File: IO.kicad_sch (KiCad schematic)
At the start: 0 parts

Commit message: Transformation in progress
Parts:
- added C4, C5: 4.7nF, Capacitor_SMD:C_0805_2012Metric_Pad1.18x1.45mm_HandSolder, symbol Device:C
- added C6, C7, C8, C9: 0.1μF, symbol Device:C
- added J11: Stop, JST-XH-4A:CONN_B4B-XH-A_JST, symbol JST-XH-4A:B4B-XH-A
- added J6: Hold, JST-XH-2A:CONN_B2B-XH-A_JST, symbol JST-XH-2A:B2B-XH-A
- added J7: X limit, JST-XH-3A:CONN_B3B-XH-A_JST, symbol JST-XH-3A:B3B-XH-A
- added J8: Y limit, JST-XH-3A:CONN_B3B-XH-A_JST, symbol JST-XH-3A:B3B-XH-A
- added R1, R2, R3, R4: 1k, Resistor_SMD:R_0805_2012Metric_Pad1.20x1.40mm_HandSolder, symbol Device:R
- added R10, R11, R12, R9: 100, symbol Device:R
- added R13, R14, R15, R16: 10, symbol Device:R
- added R6: 200, Resistor_SMD:R_0805_2012Metric_Pad1.20x1.40mm_HandSolder, symbol Device:R
- added R7: 1.2k, Resistor_SMD:R_0805_2012Metric_Pad1.20x1.40mm_HandSolder, symbol Device:R
- added SW1: Hold, Button_Switch_THT:SW_SPST_Omron_B3F-40xx, symbol Switch:SW_Push
- added SW2: Run, Button_Switch_THT:SW_SPST_Omron_B3F-40xx, symbol Switch:SW_Push
- added SW3: M1, Button_Switch_THT:SW_SPST_Omron_B3F-40xx, symbol Switch:SW_Push
- added SW4: M2, Button_Switch_THT:SW_SPST_Omron_B3F-40xx, symbol Switch:SW_Push
- added U1: SN74LV125ADR, SN74LV125ADR:SOIC127P600X175-14N, symbol SN74LV125:SN74LV125ADR
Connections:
- new net: R16.1, SW4.2
- new net: R13.2, SW1.2
- new net: R15.1, SW3.2
- new net: R14.2, SW2.2
- new net +5V: U1.1 (1~OE), U1.10 (3~OE), U1.4 (2~OE)
- new net 3.3V: J7.2, R13.1, R14.1, R15.2, R16.2, R6.2, R7.2, U1.14 (VCC)
- new net GND: C4.1, C5.1, C6.1, C7.1, C8.2, C9.2, J11.1, J6.1, J7.1, J8.1, R1.2, R2.2, R3.1, R4.1, U1.7 (GND)
- new net GPIO15: U1.9 (3A)
- new net GPIO2: U1.5 (2A)
- new net GPIO32: C5.2, J8.3, R7.1
- new net GPIO33: J7.3
- new net GPIO34: R10.2
- new net GPIO35: R9.2
- new net GPIO36: R12.2
- new net GPIO39: R11.2
- new net GPIO4: U1.2 (1A)
- new net Hold: C6.2, J6.2, R1.1, R9.1, SW1.1
- new net L_ALARM: J11.4, U1.8 (3Y)
- new net L_HOLD: J11.3, U1.6 (2Y)
- new net L_RUN: J11.2, U1.3 (1Y)
- new net M1: C8.1, R11.1, R3.2, SW3.1
- new net M2: C9.1, R12.1, R4.2, SW4.1
- new net Run: C7.2, R10.1, R2.1, SW2.1
- new net VH: C4.2, J8.2, R6.1
- no-connect marks 0 -> 3

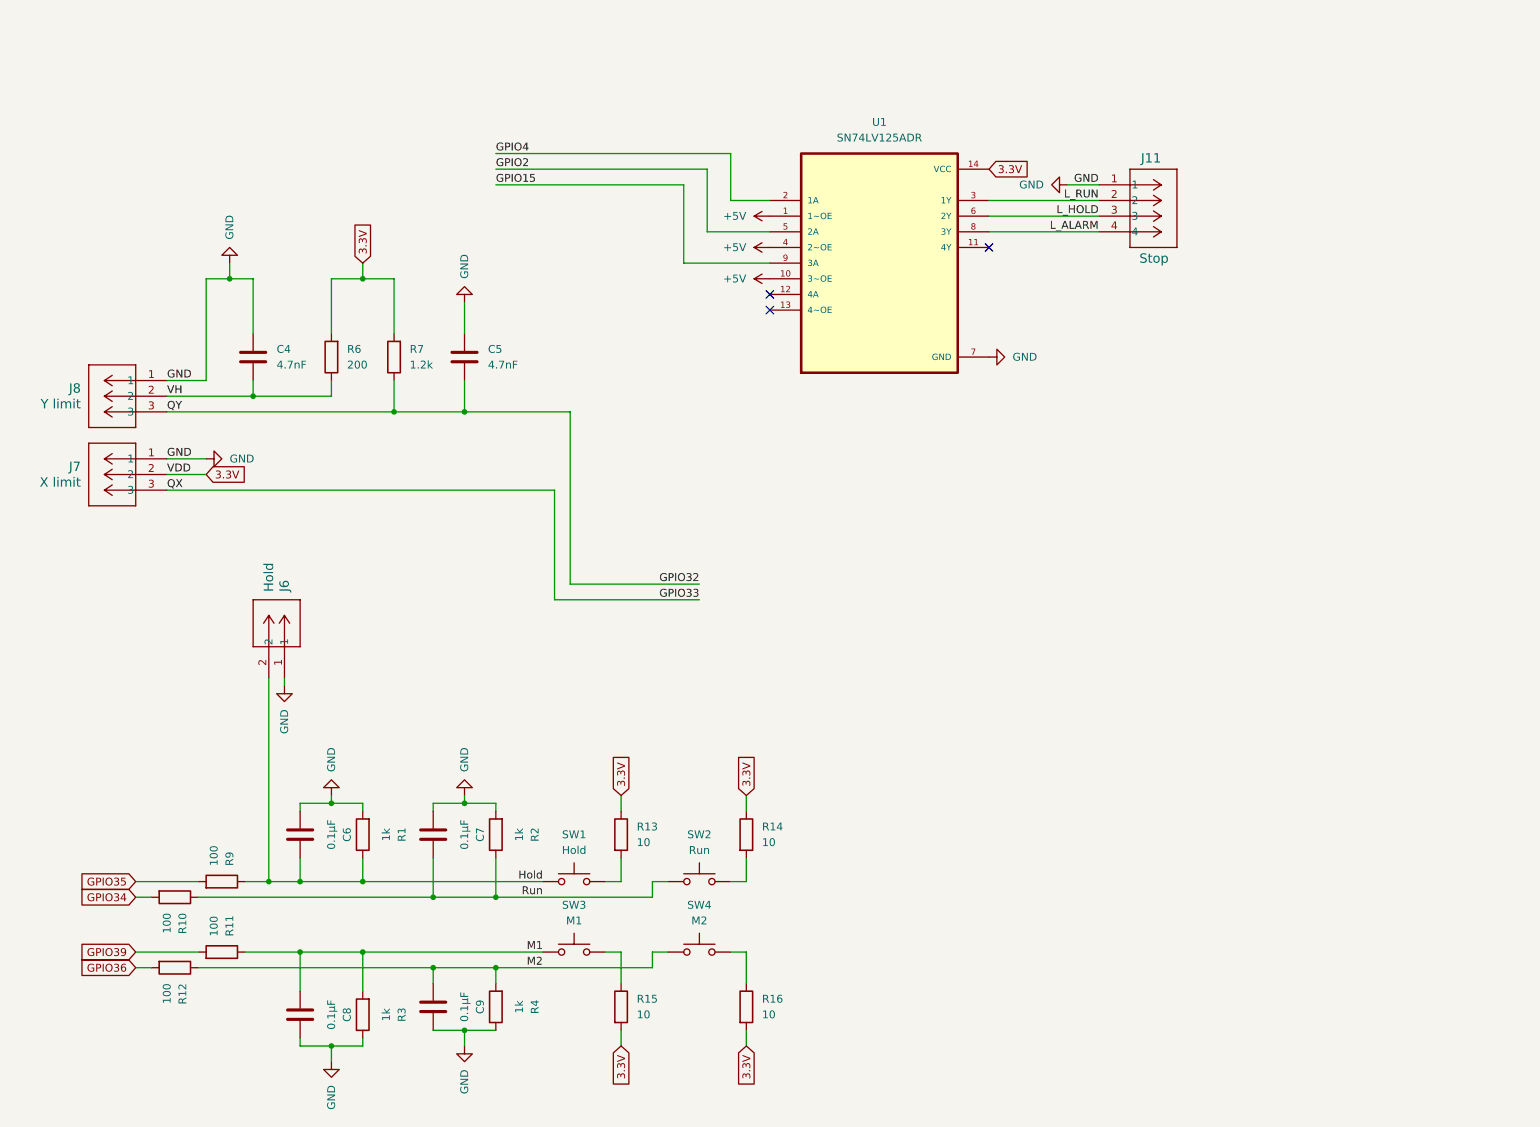
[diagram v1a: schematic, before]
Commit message: Finalization v2.0
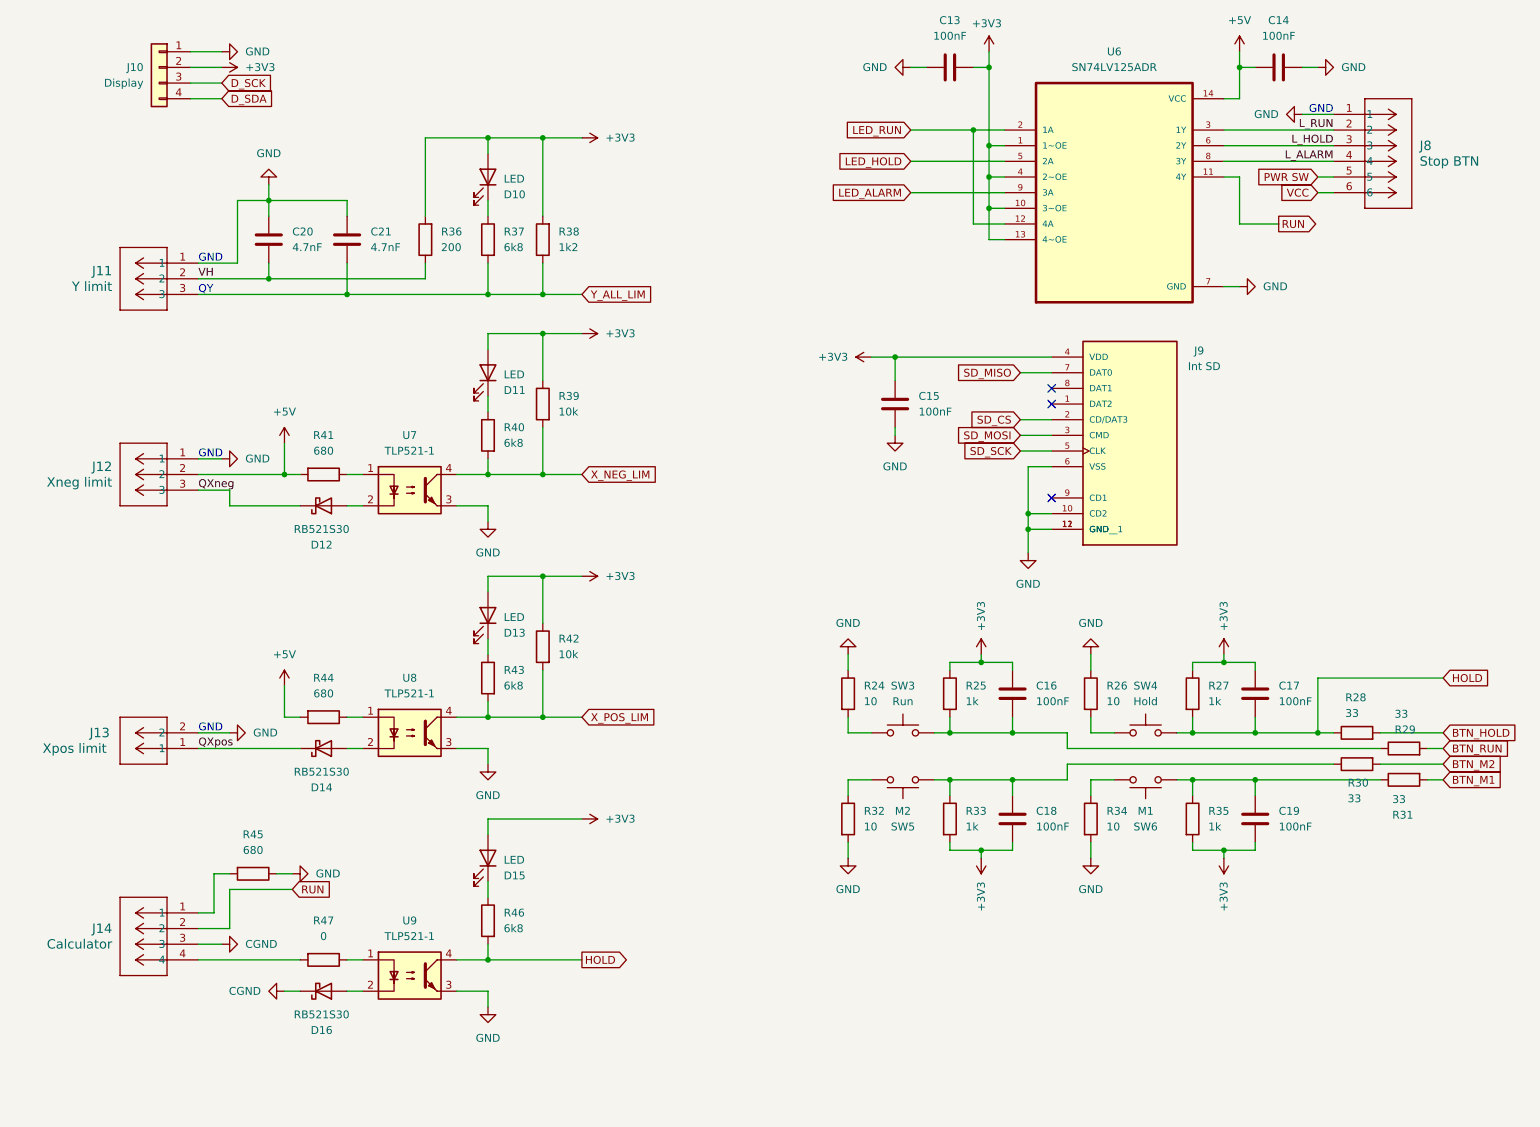
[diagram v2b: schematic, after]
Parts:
- removed C6, C7, C8, C9: 0.1μF, symbol Device:C
- removed J11: Stop, JST-XH-4A:CONN_B4B-XH-A_JST, symbol JST-XH-4A:B4B-XH-A
- removed J6: Hold, JST-XH-2A:CONN_B2B-XH-A_JST, symbol JST-XH-2A:B2B-XH-A
- removed R1, R2, R3, R4: 1k, Resistor_SMD:R_0805_2012Metric_Pad1.20x1.40mm_HandSolder, symbol Device:R
- removed R13, R14, R15, R16: 10, symbol Device:R
- added C13, C14, C15, C16, C17, C18, C19: 100nF, Capacitor_SMD:C_0805_2012Metric_Pad1.18x1.45mm_HandSolder, symbol Device:C
- added D10, D11, D13, D15: LED, LED_SMD:LED_0603_1608Metric, symbol Device:LED
- added D12, D14, D16: RB521S30, Diode_SMD:D_SOD-523, symbol Device:D_Schottky
- added J10: Display, Connector_PinSocket_2.54mm:PinSocket_1x04_P2.54mm_Vertical, symbol Connector_Generic:Conn_01x04
- added J13: Xpos limit, CONN_B2B-XH-A_JST, symbol JST-XH-2A:B2B-XH-A
- added J14: Calculator, JST-XH-4A:CONN_B4B-XH-A_JST, symbol JST-XH-4A:B4B-XH-A
- added J8: Stop BTN, JST-XH-6A:CONN_B6B-XH-A_JST, symbol JST-XH-6A:B6B-XH-A
- added J9: Int SD, MEM2061_01_188_00_A:GCT_MEM2061-01-188-00-A_REVA, symbol MEM2061_01_188_00_A:MEM2061-01-188-00-A_REVA
- added R24, R26, R32, R34: 10, Resistor_SMD:R_0805_2012Metric_Pad1.20x1.40mm_HandSolder, symbol Device:R
- added R25, R27, R33, R35: 1k, Resistor_SMD:R_0805_2012Metric_Pad1.20x1.40mm_HandSolder, symbol Device:R
- added R37, R40, R43, R46: 6k8, Resistor_SMD:R_0805_2012Metric_Pad1.20x1.40mm_HandSolder, symbol Device:R
- added R39, R42: 10k, Resistor_SMD:R_0805_2012Metric_Pad1.20x1.40mm_HandSolder, symbol Device:R
- added R41, R44, R45: 680, Resistor_SMD:R_0805_2012Metric_Pad1.20x1.40mm_HandSolder, symbol Device:R
- added R47: 0, Resistor_SMD:R_0805_2012Metric_Pad1.20x1.40mm_HandSolder, symbol Device:R
- added U7, U8, U9: TLP521-1, TLP521-1XSM:TLP521SM_ISO, symbol Isolator:Optocoupler_DC_PhotoNPN_AKEC
- J12: renamed from J7; value X limit -> Xneg limit
- R28: renamed from R9; value 100 -> 33; footprint (none) -> Resistor_SMD:R_0805_2012Metric_Pad1.20x1.40mm_HandSolder
- R29: renamed from R10; value 100 -> 33; footprint (none) -> Resistor_SMD:R_0805_2012Metric_Pad1.20x1.40mm_HandSolder
- R30: renamed from R12; value 100 -> 33; footprint (none) -> Resistor_SMD:R_0805_2012Metric_Pad1.20x1.40mm_HandSolder
- R31: renamed from R11; value 100 -> 33; footprint (none) -> Resistor_SMD:R_0805_2012Metric_Pad1.20x1.40mm_HandSolder
- R38: renamed from R7; value 1.2k -> 1k2
- renumbered C4 to C20, C5 to C21, J8 to J11, R6 to R36, SW2 to SW3, SW1 to SW4, SW4 to SW5, SW3 to SW6, U1 to U6
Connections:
- net GPIO4 is gone; now on net LED_RUN: U6.2 (1A)
- net +5V: now also J12.2, U6.14 (VCC), C14.1, R41.2, R44.2; no longer U6.1 (1~OE), U6.10 (3~OE), U6.4 (2~OE)
- net GND: now also C13.1, C14.2, C15.1, J10.1 (Pin_1), J13.2, J8.1, J9.10 (CD2), J9.11 (GND), J9.12 (GND__1), J9.6 (VSS), R24.1, R26.1, R32.2, R34.2, R45.1, U7.3, U8.3, U9.3
- net L_ALARM: now also J8.4
- net L_HOLD: now also J8.3
- net L_RUN: now also J8.2
- net at SW5.2: now also R32.1
- net at SW4.2: now also R26.2
- net at SW6.2: now also R34.1
- net at SW3.2: now also R24.2
- net RUN: now reaches U6.11 (4Y)
- net RUN: now also J14.2
- net LED_RUN: now reaches U6.12 (4A)
- net +3V3: now reaches U6.13 (4~OE)
- net +3V3: now also R36.2, R38.2, U6.1 (1~OE), U6.10 (3~OE), U6.4 (2~OE), C13.2, C15.2, C16.2, C17.2, C18.1, C19.1, D10.2 (A), D11.2 (A), D13.2 (A), D15.2 (A), J10.2 (Pin_2), J9.4 (VDD), R25.1, R27.1, R33.2, R35.2, R39.1, R42.1
- removed net 3.3V: J12.2, R36.2, R38.2, U6.14 (VCC)
- net GPIO15 renamed LED_ALARM
- net GPIO2 renamed LED_HOLD
- net GPIO32 renamed Y_ALL_LIM
- net Y_ALL_LIM: now also R37.2
- net GPIO33 renamed QXneg
- net QXneg: now also D12.1 (K)
- net GPIO34 renamed BTN_RUN
- net GPIO35 renamed BTN_HOLD
- net GPIO36 renamed BTN_M2
- net GPIO39 renamed BTN_M1
- net Hold renamed HOLD
- net HOLD: now also C17.1, R27.2, R46.2, U9.4
- net M1: no longer names the net of R31.1, SW6.1
- net M1: now also C19.2, R35.1
- net M2: no longer names the net of R30.1, SW5.1
- net M2: now also C18.2, R33.1
- net Run: no longer names the net of R29.1, SW3.1
- net Run: now also C16.1, R25.2
- new net: D13.1 (K), R43.1
- new net: D11.1 (K), R40.1
- new net: R44.1, U8.1
- new net: D10.1 (K), R37.1
- new net: R41.1, U7.1
- new net: D12.2 (A), U7.2
- new net: R47.1, U9.1
- new net: J14.4, R47.2
- new net: D14.2 (A), U8.2
- new net: D15.1 (K), R46.1
- new net: D16.2 (A), U9.2
- new net: J14.1, R45.2
- new net CGND: D16.1 (K), J14.3
- new net D_SCK: J10.3 (Pin_3)
- new net D_SDA: J10.4 (Pin_4)
- new net PWR SW: J8.5
- new net QXpos: D14.1 (K), J13.1
- new net SD_CS: J9.2 (CD/DAT3)
- new net SD_MISO: J9.7 (DAT0)
- new net SD_MOSI: J9.3 (CMD)
- new net SD_SCK: J9.5 (CLK)
- new net VCC: J8.6
- new net X_NEG_LIM: R39.2, R40.2, U7.4
- new net X_POS_LIM: R42.2, R43.2, U8.4
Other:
- note added: "GND"
- note added: "QY"
- moved on the sheet: C20, C21, J11, J12, R28, R29, R30, R31, R36, R38, SW3, SW4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
